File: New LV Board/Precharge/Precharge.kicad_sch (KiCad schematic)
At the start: 28 parts, among them Q1 BSS214NW, Q2 MPSA42, Q4 IRLML5203, U1 LM2903, U2 Optocoupler, U3 NE555P, U4 LR8N3-G

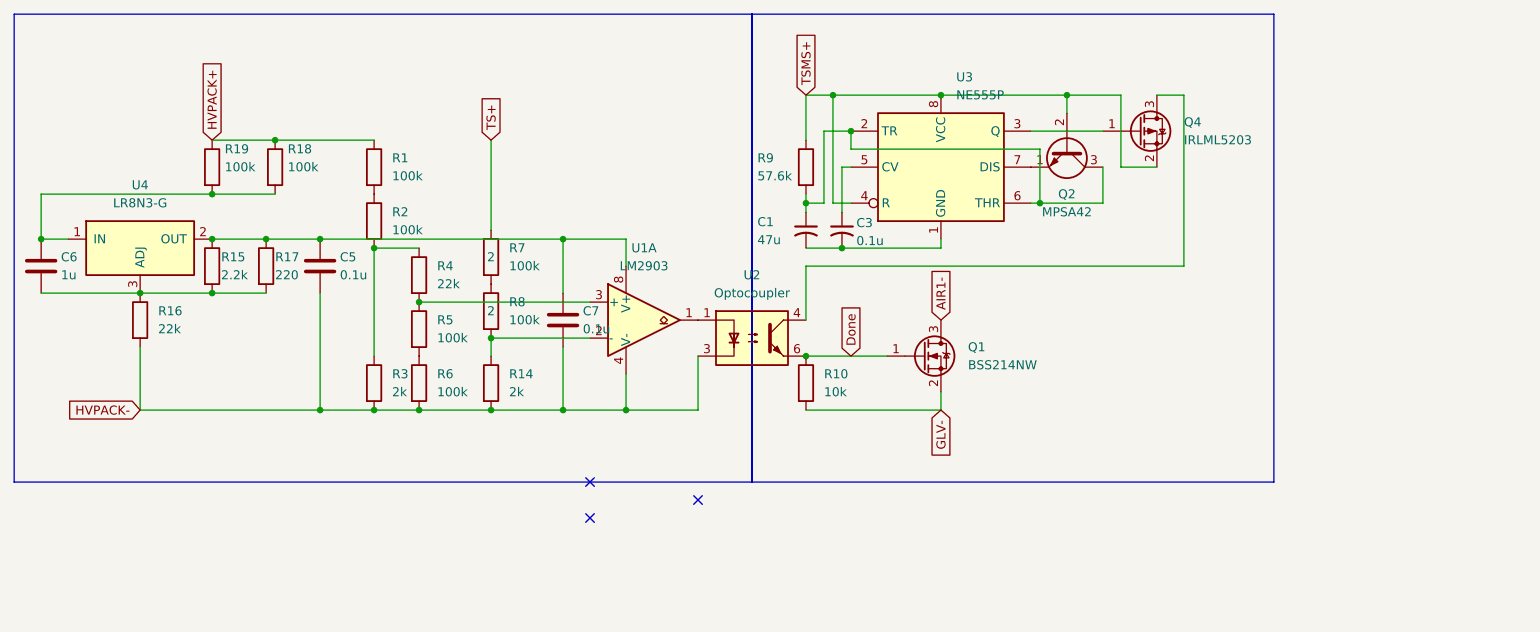
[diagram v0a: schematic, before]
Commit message: Precharge work
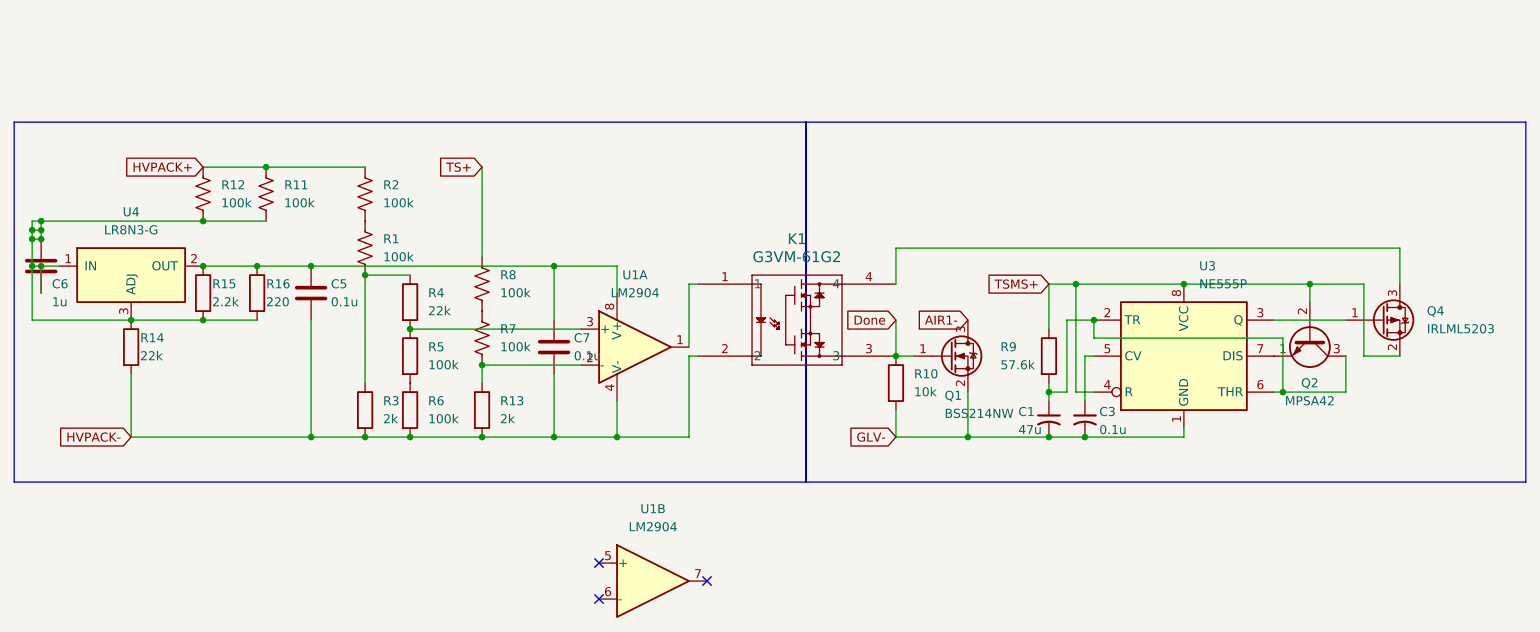
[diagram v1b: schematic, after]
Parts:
- removed R1, R18, R19, R2, R7, R8: 100k, Resistor_THT:R_Axial_DIN0411_L9.9mm_D3.6mm_P7.62mm_Vertical, symbol Device:R
- removed R17: 220, Resistor_THT:R_Axial_DIN0411_L9.9mm_D3.6mm_P7.62mm_Vertical, symbol Device:R
- removed U1: LM2903, Package_DIP:DIP-8_W7.62mm, symbol Comparator:LM2903
- removed U2: Optocoupler, Package_SO:SOIC-4_4.55x3.7mm_P2.54mm, symbol Isolator:Optocoupler_DC_PhotoNPN_AKEC
- added K1: G3VM-61G2, Precharge:G-SOP4_OMR, symbol Precharge:G3VM-61G2
- added R1, R11, R12, R2, R7, R8: 100k, Resistor_THT:R_Axial_DIN0516_L15.5mm_D5.0mm_P5.08mm_Vertical, symbol Device:R_US
- added R13: 2k, Resistor_THT:R_Axial_DIN0207_L6.3mm_D2.5mm_P2.54mm_Vertical, symbol Device:R
- added U1: LM2904, Package_DIP:DIP-8_W7.62mm, symbol Amplifier_Operational:LM2904
- C1: Link (none) -> https://www.digikey.com/en/products/detail/samsung-electro-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; Name (none) -> 47u Cap
- C3: footprint Capacitor_SMD:C_1210_3225Metric_Pad1.33x2.70mm_HandSolder -> Capacitor_SMD:C_1206_3216Metric_Pad1.33x1.80mm_HandSolder; Link (none) -> https://www.digikey.com/en/products/detail/samsung-electro-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; Name (none) -> 0.1u Cap
- C5, C7: footprint (none) -> Capacitor_SMD:C_1206_3216Metric_Pad1.33x1.80mm_HandSolder; Link (none) -> https://www.digikey.com/en/products/detail/samsung-electro-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; Name (none) -> 0.1u Cap
- C6: footprint (none) -> Capacitor_SMD:C_1206_3216Metric_Pad1.33x1.80mm_HandSolder; Link (none) -> https://www.digikey.com/en/products/detail/samsung-electro-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; Name (none) -> 1u Cap
- Q1: Link (none) -> https://www.digikey.at/en/products/detail/infineon-technolo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; Name (none) -> NMOS
- Q2: Link (none) -> https://www.digikey.com/en/products/detail/onsemi/MPSA42/32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; Name (none) -> PNP Transistor
- Q4: Link (none) -> https://www.digikey.com/en/products/detail/infineon-technol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; Name (none) -> PMOS
- R10: footprint Resistor_THT:R_Axial_DIN0411_L9.9mm_D3.6mm_P7.62mm_Vertical -> Resistor_THT:R_Axial_DIN0207_L6.3mm_D2.5mm_P2.54mm_Vertical; Name (none) -> 10k Resistor
- R14: value 2k -> 22k; footprint Resistor_THT:R_Axial_DIN0411_L9.9mm_D3.6mm_P7.62mm_Vertical -> Resistor_THT:R_Axial_DIN0207_L6.3mm_D2.5mm_P2.54mm_Vertical; Name (none) -> 22k Resistor
- R15: footprint Resistor_THT:R_Axial_DIN0411_L9.9mm_D3.6mm_P7.62mm_Vertical -> Resistor_THT:R_Axial_DIN0207_L6.3mm_D2.5mm_P2.54mm_Vertical; Name (none) -> 2.2k Resistor
- R16: value 22k -> 220; footprint Resistor_THT:R_Axial_DIN0411_L9.9mm_D3.6mm_P7.62mm_Vertical -> Resistor_THT:R_Axial_DIN0207_L6.3mm_D2.5mm_P2.54mm_Vertical; Name (none) -> 220 Resistor
- R3: footprint Resistor_THT:R_Axial_DIN0411_L9.9mm_D3.6mm_P7.62mm_Vertical -> Resistor_THT:R_Axial_DIN0207_L6.3mm_D2.5mm_P2.54mm_Vertical; Name (none) -> 2k Resistor
- R4: footprint Resistor_THT:R_Axial_DIN0411_L9.9mm_D3.6mm_P7.62mm_Vertical -> Resistor_THT:R_Axial_DIN0207_L6.3mm_D2.5mm_P2.54mm_Vertical; Name (none) -> 22k Resistor
- R5, R6: footprint Resistor_THT:R_Axial_DIN0411_L9.9mm_D3.6mm_P7.62mm_Vertical -> Resistor_THT:R_Axial_DIN0207_L6.3mm_D2.5mm_P2.54mm_Vertical; Name (none) -> 100k Resistor
- R9: footprint Resistor_THT:R_Axial_DIN0411_L9.9mm_D3.6mm_P7.62mm_Vertical -> Resistor_THT:R_Axial_DIN0207_L6.3mm_D2.5mm_P2.54mm_Vertical; Name (none) -> 57.6k Resistor
- U3: Link (none) -> https://www.digikey.com/en/products/detail/texas-instrument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; Name (none) -> 555 Timer
- U4: Link (none) -> https://www.digikey.com/en/products/detail/microchip-techno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; Name (none) -> Linear Voltage Regulator
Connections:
- net Done: now also K1.3
- net GLV-: now also C1.2, C3.2, U3.1 (GND)
- net HVPACK+: now also R11.1, R12.1, R2.1
- net HVPACK-: now also K1.2, R13.2, U1.4 (V-); no longer R16.2
- net TS+: now also R8.1
- net at R3.1, R4.1: now also R1.2
- net at R4.2, R5.1: now also U1.3 (+)
- net at C6.1, U4.1 (IN): now also C6.2, R14.1, R15.2, R16.2, U4.3 (ADJ), R11.2, R12.2
- net at C5.1, C7.1, R15.1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: now also R16.1, U1.8 (V+)
- net at Q4.3 (D): now also K1.4
- new net: K1.1, U1.1
- new net: R1.1, R2.2
- new net: R13.1, R7.2, U1.2 (-)
- new net: R7.1, R8.2
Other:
- moved on the sheet: C1, C3, C5, C7, Q1, Q2, Q4, R10, R15, R3, R4, R6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
